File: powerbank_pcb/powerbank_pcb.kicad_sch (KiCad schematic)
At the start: 18 parts, among them SW1 TS-1002S-04526C, U1 TP4366E

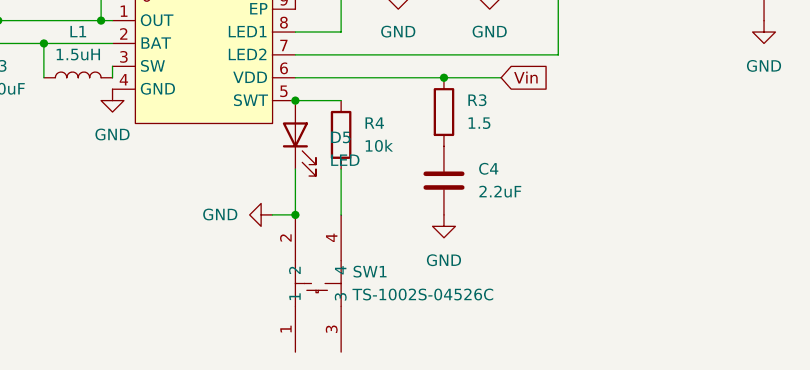
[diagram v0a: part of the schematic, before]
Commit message: update
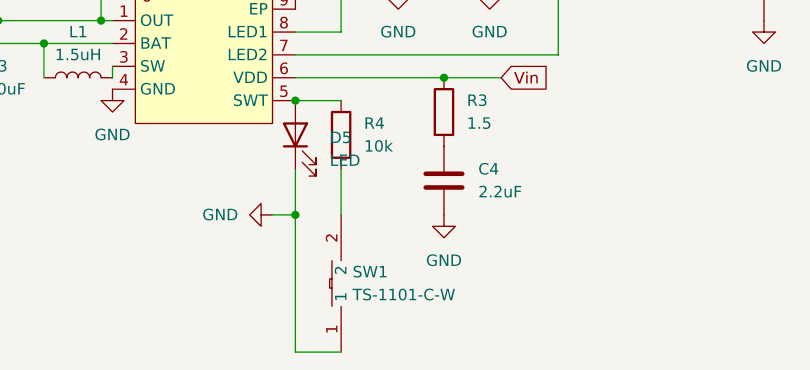
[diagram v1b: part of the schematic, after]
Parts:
- removed SW1: TS-1002S-04526C, Button_Switch_SMD:Nidec_Copal_CAS-120A, symbol easyeda2kicad:TS-1002S-04526C
- added SW1: TS-1101-C-W, easyeda2kicad:SW-SMD_L6.0-W3.3-LS8.0, symbol easyeda2kicad:TS-1101-C-W
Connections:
- net GND: now also SW1.1
- net at R4.2: now also SW1.2
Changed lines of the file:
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@@
+	)
+	(junction
+		(at 132.08 30.48)
+		(diameter 0)
+		(color 0 0 0 0)
+	)
+	(junction
+		(at 142.24 30.48)
+		(diameter 0)
+		(color 0 0 0 0)
+	)
+	(junction
+		(at 120.65 53.34)
+		(diameter 0)
+		(color 0 0 0 0)
+	)
+	(junction
+		(at 92.71 30.48)
+		(diameter 0)
+		(color 0 0 0 0)
+	)
+	(junction
+		(at 99.06 44.45)
+		(diameter 0)
+		(color 0 0 0 0)
+	)
+	(junction
+		(at 82.55 46.99)
+		(diameter 0)
+		(color 0 0 0 0)
 	)
 	(junction
@@
 	)
 	(junction
-		(at 132.08 30.48)
-		(diameter 0)
-		(color 0 0 0 0)
-	)
-	(junction
-		(at 142.24 30.48)
-		(diameter 0)
-		(color 0 0 0 0)
-	)
-	(junction
-		(at 120.65 53.34)
-		(diameter 0)
-		(color 0 0 0 0)
-	)
-	(junction
-		(at 92.71 30.48)
-		(diameter 0)
-		(color 0 0 0 0)
-	)
-	(junction
-		(at 99.06 44.45)
-		(diameter 0)
-		(color 0 0 0 0)
-	)
-	(junction
-		(at 82.55 46.99)
-		(diameter 0)
-		(color 0 0 0 0)
-	)
-	(junction
 		(at 137.16 50.8)
 		(diameter 0)
@@
 	(wire
 		(pts
+			(xy 120.65 81.28) (xy 120.65 66.04)
+		)
+		(stroke
+			(width 0)
+			(type default)
+		)
+	)
+	(wire
+		(pts
 			(xy 142.24 29.21) (xy 142.24 30.48)
 		)
@@
 		(pts
 			(xy 87.63 38.1) (xy 87.63 44.45)
+		)
+		(stroke
+			(width 0)
+			(type default)
+		)
+	)
+	(wire
+		(pts
+			(xy 125.73 81.28) (xy 120.65 81.28)
 		)
 		(stroke
@@
 	)
 	(symbol
+		(lib_id "easyeda2kicad:TS-1101-C-W")
+		(at 125.73 73.66 90)
+		(unit 1)
+		(exclude_from_sim no)
+		(in_bom yes)
+		(on_board yes)
+		(dnp no)
+		(fields_autoplaced yes)
+		(property "Reference" "SW1"
+			(at 127 72.3899 90)
+			(effects
+				(font
+					(size 1.27 1.27)
+				)
+				(justify right)
+			)
+		)
+		(property "Value" "TS-1101-C-W"
+			(at 127 74.9299 90)
+			(effects
+				(font
+					(size 1.27 1.27)
+				)
+				(justify right)
+			)
+		)
+		(property "Footprint" "easyeda2kicad:SW-SMD_L6.0-W3.3-LS8.0"
+			(at 133.35 73.66 0)
+			(effects
+				(font
+					(size 1.27 1.27)
+				)
+				(hide yes)
+			)
+		)
+		(property "Datasheet" ""
+			(at 125.73 73.66 0)
+			(effects
+				(font
+					(size 1.27 1.27)
+				)
+				(hide yes)
+			)
+		)
+		(property "Description" ""
+			(at 125.73 73.66 0)
+			(effects
+				(font
+					(size 1.27 1.27)
+				)
+				(hide yes)
+			)
+		)
+		(property "LCSC Part" "C318938"
+			(at 135.89 73.66 0)
+			(effects
+				(font
+					(size 1.27 1.27)
+				)
+				(hide yes)
+			)
+		)
+		(pin "2"
+		)
+		(pin "1"
+		)
+		(instances
+			(project ""
+				(path "/332d7591-23c8-46ee-88ac-d4cbe8afaa76"
+					(reference "SW1")
+					(unit 1)
+				)
+			)
+		)
+	)
+	(symbol
 		(lib_id "power:GND")
 		(at 92.71 30.48 180)
@@
 					(unit 1)
 				)
-			)
-		)
-	)
-	(symbol
-		(lib_id "easyeda2kicad:TS-1002S-04526C")
-		(at 123.19 73.66 90)
-		(unit 1)
-		(exclude_from_sim no)
-		(in_bom yes)
-		(on_board yes)
-		(dnp no)
-		(fields_autoplaced yes)
-		(property "Reference" "SW1"
-			(at 127 72.3899 90)
-			(effects
-				(font
-					(size 1.27 1.27)
-				)
-				(justify right)
-			)
-		)
-		(property "Value" "TS-1002S-04526C"
-			(at 127 74.9299 90)
-			(effects
-				(font
-					(size 1.27 1.27)
-				)
-				(justify right)
-			)
-		)
-		(property "Footprint" "Button_Switch_SMD:Nidec_Copal_CAS-120A"
-			(at 133.35 73.66 0)
-			(effects
-				(font
-					(size 1.27 1.27)
-				)
-				(hide yes)
-			)
-		)
-		(property "Datasheet" "https://lcsc.com/product-detail/Tactile-Switches_XUNPU-TS-1002S-04526C_C455109.html"
-			(at 135.89 73.66 0)
-			(effects
-				(font
-					(size 1.27 1.27)
-				)
-				(hide yes)
-			)
-		)
-		(property "Description" ""
-			(at 123.19 73.66 0)
-			(effects
-				(font
-					(size 1.27 1.27)
-				)
-				(hide yes)
-			)
-		)
-		(property "LCSC Part" "C455109"
-			(at 138.43 73.66 0)
-			(effects
-				(font
-					(size 1.27 1.27)
-				)
-				(hide yes)
-			)
-		)
-		(pin "2"
-		)
-		(pin "4"
-		)
-		(pin "1"
-		)
-		(pin "3"
-		)
-		(instances
-			(project ""
-				(path "/332d7591-23c8-46ee-88ac-d4cbe8afaa76"
-					(reference "SW1")
-					(unit 1)
-				)
